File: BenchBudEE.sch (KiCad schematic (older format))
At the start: 0 parts

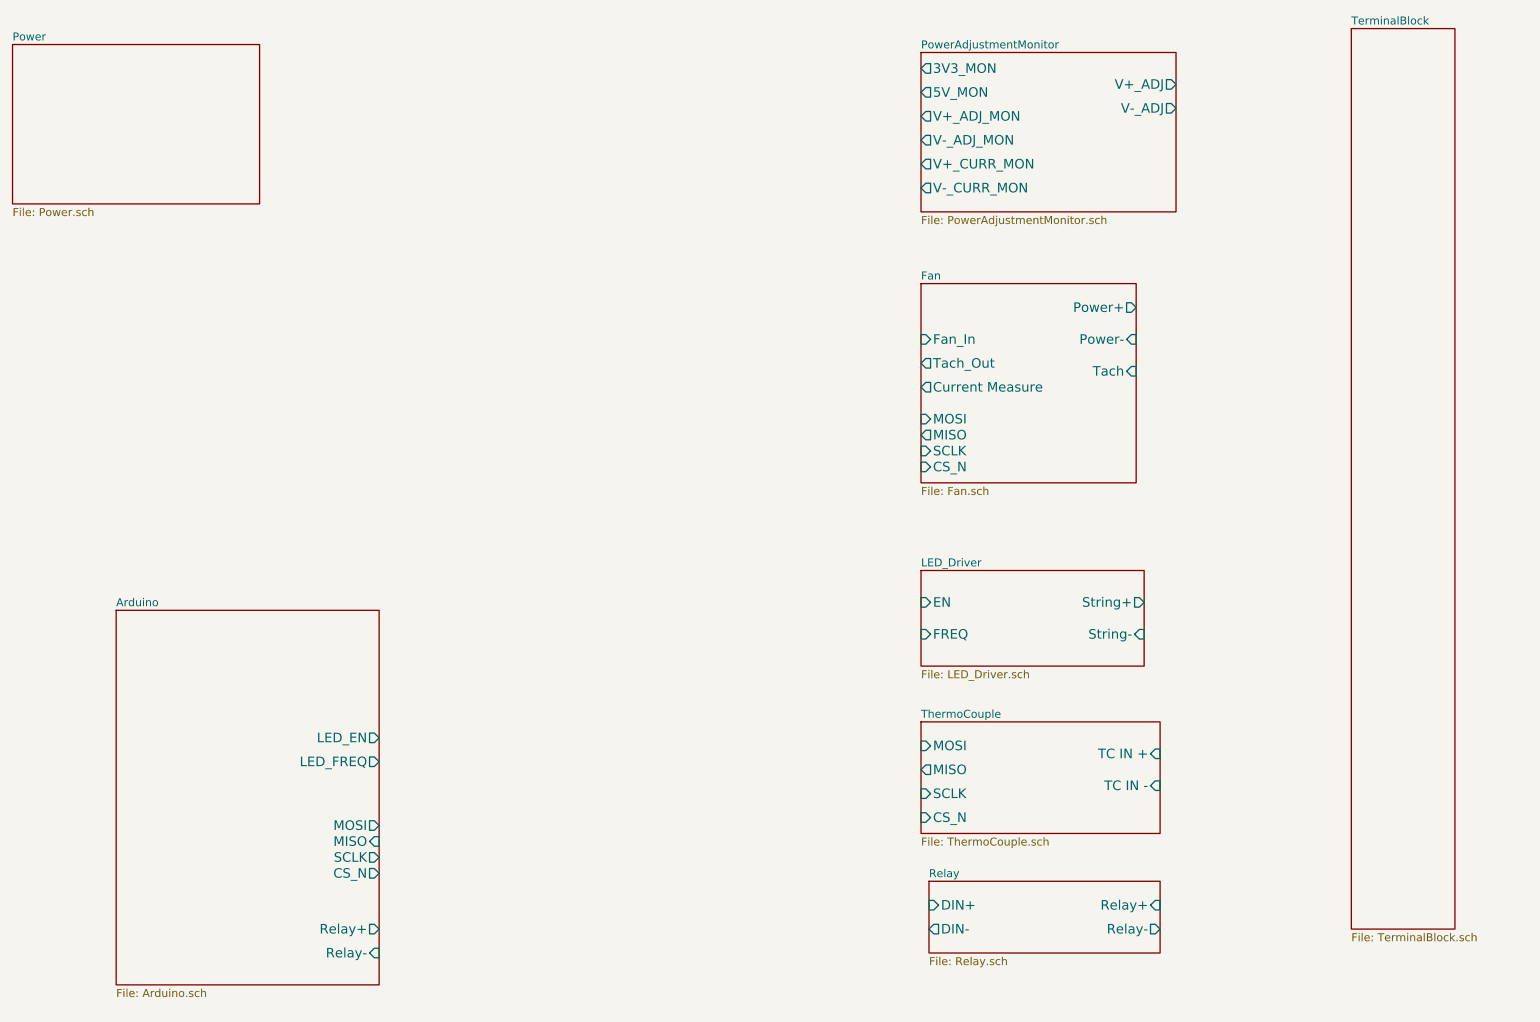
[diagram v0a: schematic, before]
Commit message: Hooked up top level schematic
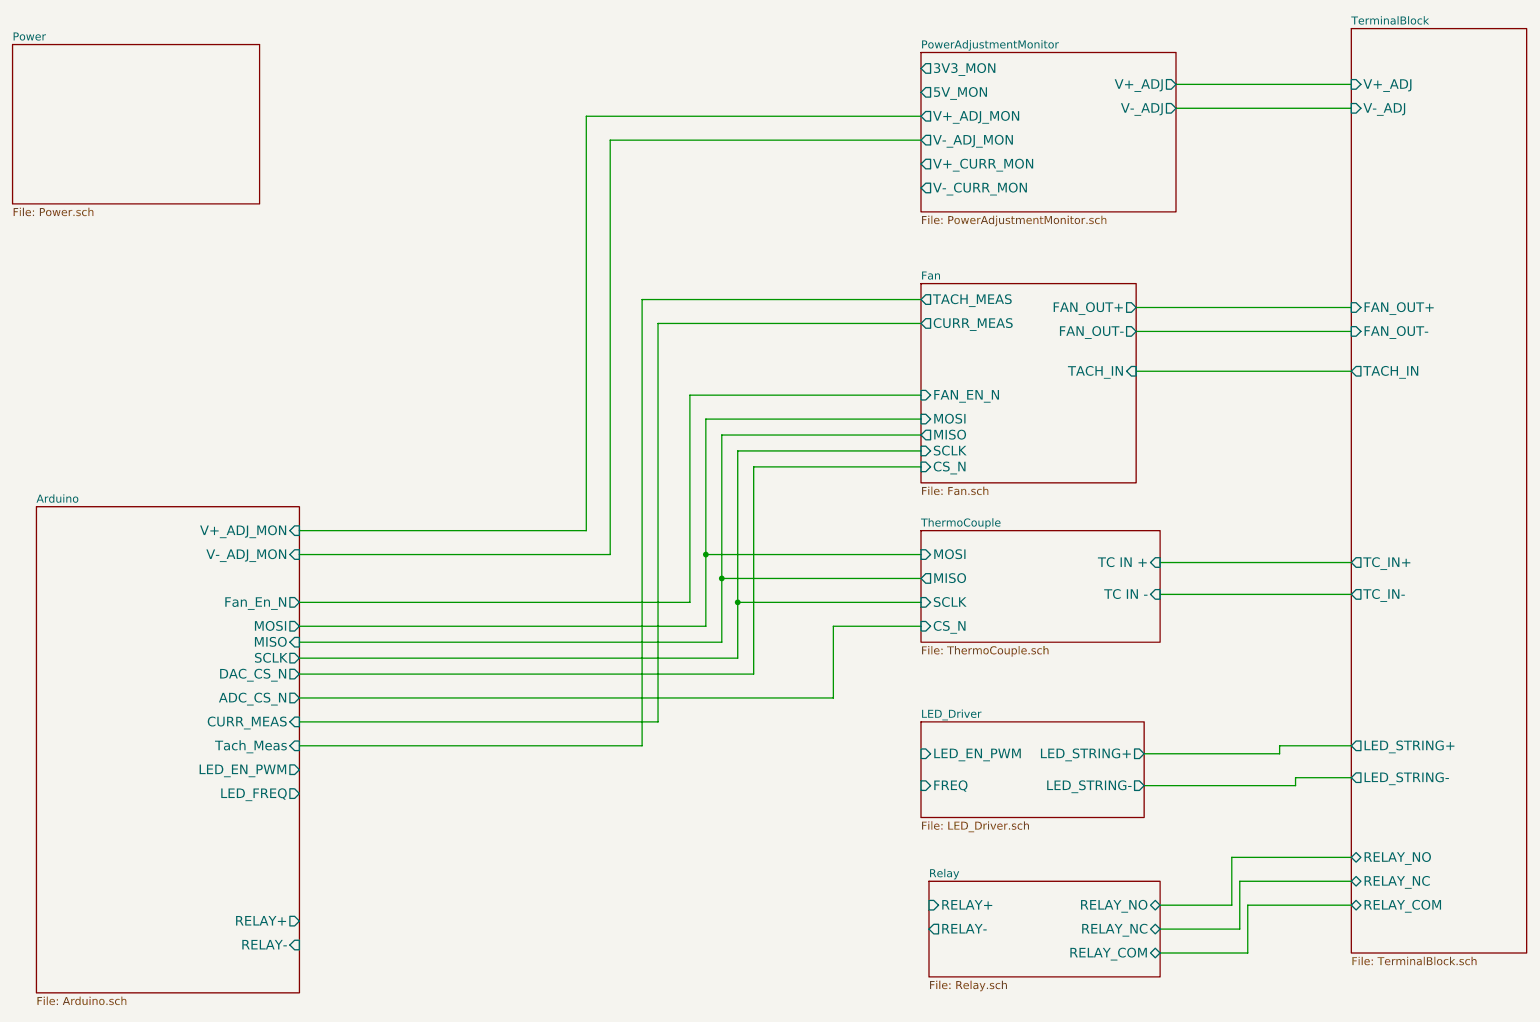
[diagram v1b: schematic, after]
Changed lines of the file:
@@
 $EndDescr
 $Sheet
-S 2200 4750 1650 2350
-U 52ED1A8D
-F0 "Arduino" 50
-F1 "Arduino.sch" 50
-F2 "Relay+" O R 3850 6750 60
-F3 "Relay-" I R 3850 6900 60
-F4 "MOSI" O R 3850 6100 60
-F5 "MISO" I R 3850 6200 60
-F6 "SCLK" O R 3850 6300 60
-F7 "CS_N" O R 3850 6400 60
-F8 "LED_EN" O R 3850 5550 60
-F9 "LED_FREQ" O R 3850 5700 60
-$EndSheet
-$Sheet
-S 7250 5450 1500 700
+S 7250 4250 1500 700
 U 52ED1AE1
 F0 "ThermoCouple" 50
 F1 "ThermoCouple.sch" 50
-F2 "TC IN +" I R 8750 5650 60
-F3 "TC IN -" I R 8750 5850 60
-F4 "MOSI" I L 7250 5600 60
-F5 "MISO" O L 7250 5750 60
-F6 "SCLK" I L 7250 5900 60
-F7 "CS_N" I L 7250 6050 60
-$EndSheet
-$Sheet
-S 7300 6450 1450 450
+F2 "TC IN +" I R 8750 4450 60
+F3 "TC IN -" I R 8750 4650 60
+F4 "MOSI" I L 7250 4400 60
+F5 "MISO" O L 7250 4550 60
+F6 "SCLK" I L 7250 4700 60
+F7 "CS_N" I L 7250 4850 60
+$EndSheet
+$Sheet
+S 7300 6450 1450 600
 U 52ED1B00
 F0 "Relay" 50
 F1 "Relay.sch" 50
-F2 "DIN+" I L 7300 6600 60
-F3 "DIN-" O L 7300 6750 60
-F4 "Relay+" I R 8750 6600 60
-F5 "Relay-" O R 8750 6750 60
+F2 "RELAY_NO" B R 8750 6600 60
+F3 "RELAY_NC" B R 8750 6750 60
+F4 "RELAY_COM" B R 8750 6900 60
+F5 "RELAY+" I L 7300 6600 60
+F6 "RELAY-" O L 7300 6750 60
 $EndSheet
 $Sheet
@@
 $EndSheet
 $Sheet
-S 7250 4500 1400 600
+S 7250 5450 1400 600
 U 52ED1B6A
 F0 "LED_Driver" 50
 F1 "LED_Driver.sch" 50
-F2 "EN" I L 7250 4700 60
-F3 "FREQ" I L 7250 4900 60
-F4 "String+" O R 8650 4700 60
-F5 "String-" I R 8650 4900 60
+F2 "FREQ" I L 7250 5850 60
+F3 "LED_EN_PWM" I L 7250 5650 60
+F4 "LED_STRING+" O R 8650 5650 60
+F5 "LED_STRING-" O R 8650 5850 60
 $EndSheet
 $Sheet
@@
 F0 "Fan" 50
 F1 "Fan.sch" 50
-F2 "Power+" O R 8600 2850 60
-F3 "Power-" I R 8600 3050 60
-F4 "Tach" I R 8600 3250 60
-F5 "Tach_Out" O L 7250 3200 60
-F6 "Fan_In" I L 7250 3050 60
-F7 "MOSI" I L 7250 3550 60
-F8 "MISO" O L 7250 3650 60
-F9 "SCLK" I L 7250 3750 60
-F10 "CS_N" I L 7250 3850 60
-F11 "Current Measure" O L 7250 3350 60
-$EndSheet
-$Sheet
-S 9950 1100 650  5650
+F2 "MOSI" I L 7250 3550 60
+F3 "MISO" O L 7250 3650 60
+F4 "SCLK" I L 7250 3750 60
+F5 "CS_N" I L 7250 3850 60
+F6 "FAN_OUT+" O R 8600 2850 60
+F7 "TACH_IN" I R 8600 3250 60
+F8 "TACH_MEAS" O L 7250 2800 60
+F9 "FAN_EN_N" I L 7250 3400 60
+F10 "CURR_MEAS" O L 7250 2950 60
+F11 "FAN_OUT-" O R 8600 3000 60
+$EndSheet
+$Sheet
+S 9950 1100 1100 5800
 U 52ED1C0B
 F0 "TerminalBlock" 50
 F1 "TerminalBlock.sch" 50
+F2 "V+_ADJ" I L 9950 1450 60
+F3 "V-_ADJ" I L 9950 1600 60
+F4 "FAN_OUT+" I L 9950 2850 60
+F5 "FAN_OUT-" I L 9950 3000 60
+F6 "TACH_IN" O L 9950 3250 60
+F7 "LED_STRING+" O L 9950 5600 60
+F8 "LED_STRING-" O L 9950 5800 60
+F9 "TC_IN+" O L 9950 4450 60
+F10 "TC_IN-" O L 9950 4650 60
+F11 "RELAY_NO" B L 9950 6300 60
+F12 "RELAY_NC" B L 9950 6450 60
+F13 "RELAY_COM" B L 9950 6600 60
 $EndSheet
 $Sheet
@@
 F9 "V-_CURR_MON" O L 7250 2100 60
 $EndSheet
+Wire Wire Line
+	9950 1450 8850 1450
+Wire Wire Line
+	8850 1600 9950 1600
+Wire Wire Line
+	9950 2850 8600 2850
+Wire Wire Line
+	8600 3000 9950 3000
+Wire Wire Line
+	9950 3250 8600 3250
+Wire Wire Line
+	8750 6600 9200 6600
+Wire Wire Line
+	9200 6600 9200 6300
+Wire Wire Line
+	9200 6300 9950 6300
+Wire Wire Line
+	8750 6750 9250 6750
+Wire Wire Line
+	9250 6750 9250 6450
+Wire Wire Line
+	9250 6450 9950 6450
+Wire Wire Line
+	8750 6900 9300 6900
+Wire Wire Line
+	9300 6900 9300 6600
+Wire Wire Line
+	9300 6600 9950 6600
+Wire Wire Line
+	3350 4250 5150 4250
+Wire Wire Line
+	5150 4250 5150 1650
+Wire Wire Line
+	5150 1650 7250 1650
+Wire Wire Line
+	3350 4400 5300 4400
+Wire Wire Line
+	5300 4400 5300 1800
+Wire Wire Line
+	5300 1800 7250 1800
+Wire Wire Line
+	5800 3400 7250 3400
+Wire Wire Line
+	5800 3400 5800 4700
+Wire Wire Line
+	5800 4700 3350 4700
+$Sheet
+S 1700 4100 1650 3050
+U 52ED1A8D
+F0 "Arduino" 50
+F1 "Arduino.sch" 50
+F2 "MOSI" O R 3350 4850 60
+F3 "MISO" I R 3350 4950 60
+F4 "SCLK" O R 3350 5050 60
+F5 "LED_FREQ" O R 3350 5900 60
+F6 "Fan_En_N" O R 3350 4700 60
+F7 "Tach_Meas" I R 3350 5600 60
+F8 "CURR_MEAS" I R 3350 5450 60
+F9 "RELAY+" O R 3350 6700 60
+F10 "RELAY-" I R 3350 6850 60
+F11 "LED_EN_PWM" O R 3350 5750 60
+F12 "V+_ADJ_MON" I R 3350 4250 60
+F13 "V-_ADJ_MON" I R 3350 4400 60
+F14 "DAC_CS_N" O R 3350 5150 60
+F15 "ADC_CS_N" O R 3350 5300 60
+$EndSheet
+Wire Wire Line
+	7250 3550 5900 3550
+Wire Wire Line
+	5900 3550 5900 4850
+Wire Wire Line
+	5900 4850 3350 4850
+Wire Wire Line
+	3350 4950 6000 4950
+Wire Wire Line
+	6000 4950 6000 3650
+Wire Wire Line
+	6000 3650 7250 3650
+Wire Wire Line
+	7250 3750 6100 3750
+Wire Wire Line
+	6100 3750 6100 5050
+Wire Wire Line
+	6100 5050 3350 5050
+Wire Wire Line
+	3350 5150 6200 5150
+Wire Wire Line
+	6200 5150 6200 3850
+Wire Wire Line
+	6200 3850 7250 3850
+Wire Wire Line
+	7250 4850 6700 4850
+Wire Wire Line
+	6700 4850 6700 5300
+Wire Wire Line
+	6700 5300 3350 5300
+Wire Wire Line
+	7250 4700 6100 4700
+Connection ~ 6100 4700
+Wire Wire Line
+	6000 4550 7250 4550
+Connection ~ 6000 4550
+Wire Wire Line
+	7250 4400 5900 4400
+Connection ~ 5900 4400
+Wire Wire Line
+	7250 2950 5600 2950
+Wire Wire Line
+	5600 2950 5600 5450
+Wire Wire Line
+	5600 5450 3350 5450
+Wire Wire Line
+	3350 5600 5500 5600
+Wire Wire Line
+	5500 5600 5500 2800
+Wire Wire Line
+	5500 2800 7250 2800
+Wire Wire Line
+	8750 4450 9950 4450
+Wire Wire Line
+	8750 4650 9950 4650
+Wire Wire Line
+	8650 5650 9500 5650
+Wire Wire Line
+	9500 5650 9500 5600
+Wire Wire Line
+	9500 5600 9950 5600
+Wire Wire Line
+	8650 5850 9600 5850
+Wire Wire Line
+	9600 5850 9600 5800
+Wire Wire Line
+	9600 5800 9950 5800
 $EndSCHEMATC
